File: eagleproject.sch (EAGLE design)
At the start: 6 parts, among them J1 RASPBERRYPI-40-PIN-GPIO_PTH, J2 XLR-3-FEMALE, J3 XLR-3-MALE

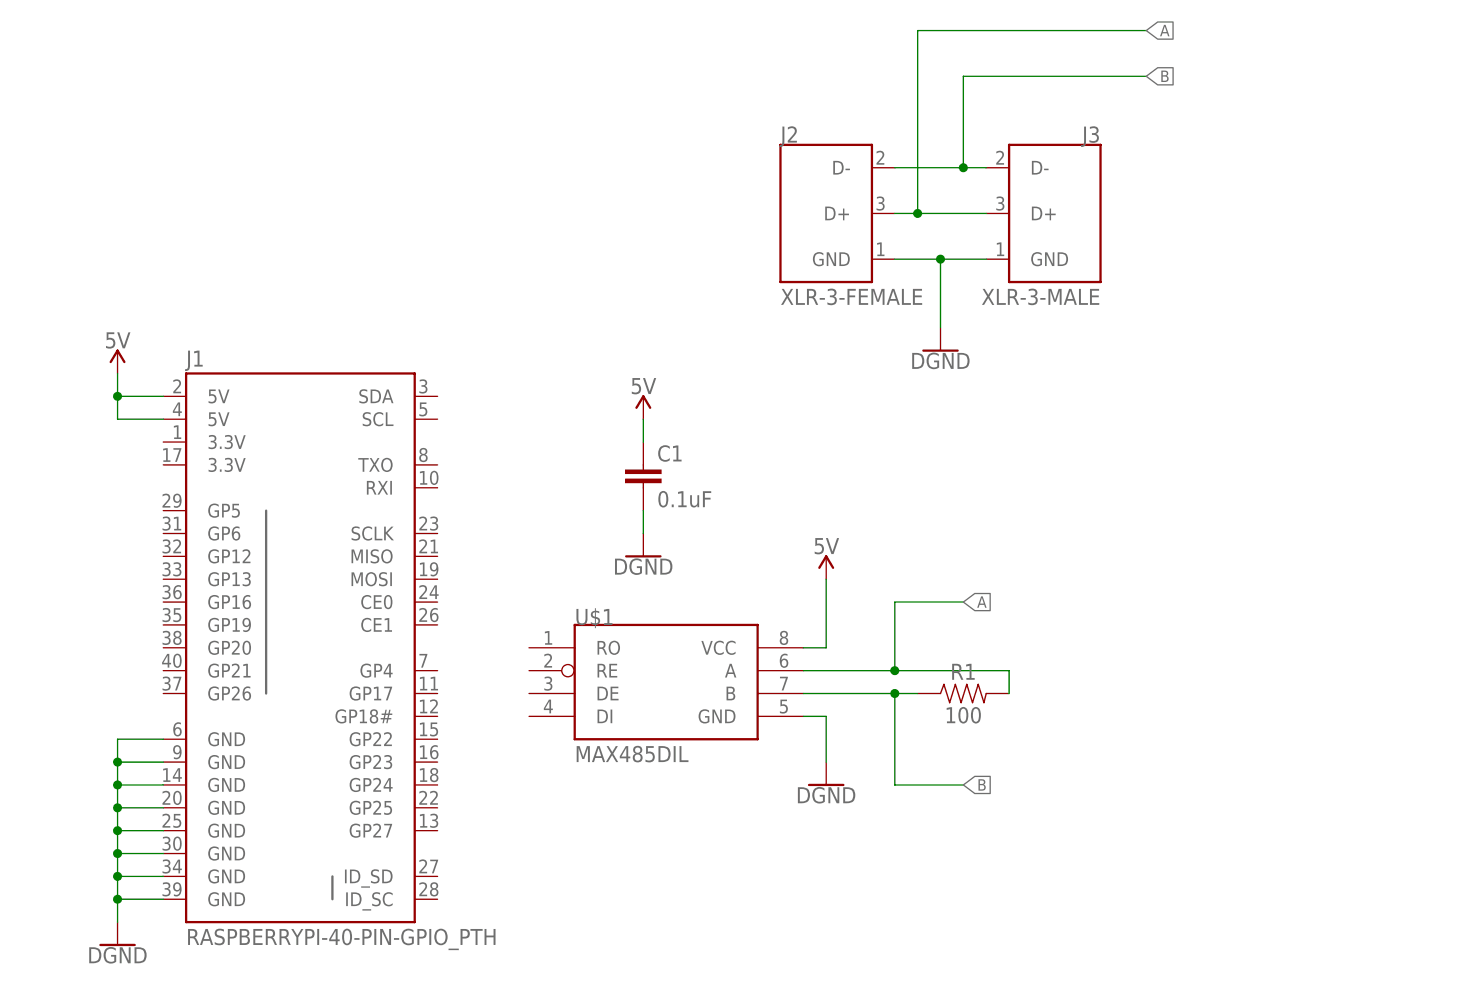
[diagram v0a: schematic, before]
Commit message: first version for manufacturing
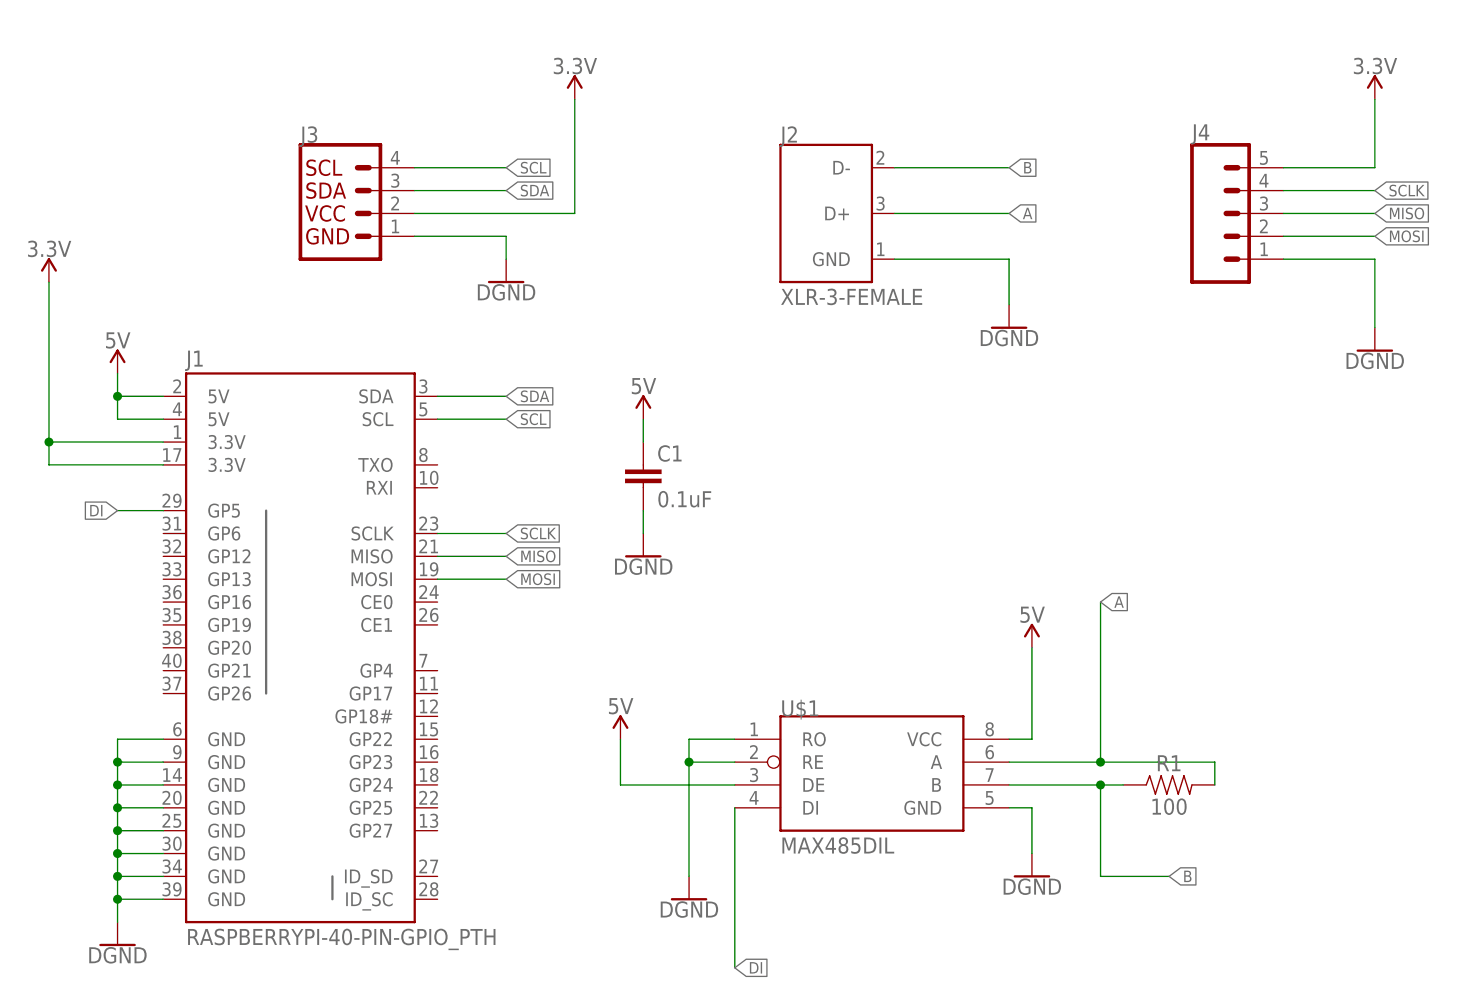
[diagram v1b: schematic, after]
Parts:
- added J4: (no value), SparkFun-Connectors:CONN_05
- J3: value XLR-3-MALE -> (none); device SparkFun-Connectors:XLR-3-MALE -> SparkFun-Connectors:I2C_STANDARD
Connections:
- new net 3.3V: J1.3.3V@1, J1.3.3V@17, J3.2, J4.5
- new net DI: J1.GP5, U$1.DI
- new net MISO: J1.MISO, J4.3
- new net MOSI: J1.MOSI, J4.2
- new net SCL: J1.SCL, J3.4
- new net SCLK: J1.SCLK, J4.4
- new net SDA: J1.SDA, J3.3
- net 5V: now also U$1.DE
- net A: no longer J3.D+
- net B: no longer J3.D-
- net GND: now also J3.1, J4.1, U$1.RE, U$1.RO; no longer J3.GND
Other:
- moved on the sheet: R1, U$1
